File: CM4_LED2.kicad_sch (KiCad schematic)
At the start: 2 parts

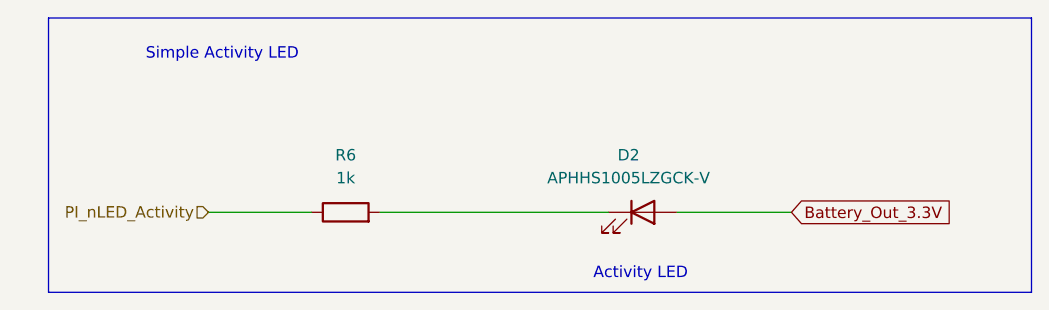
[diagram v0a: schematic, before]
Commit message: chore: Many routing changes
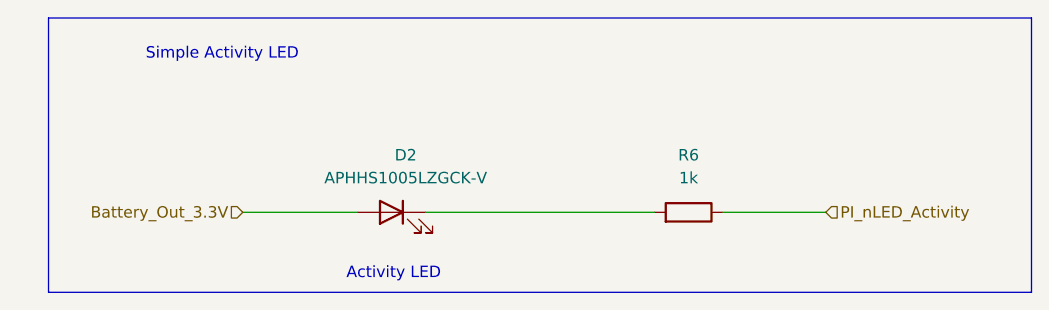
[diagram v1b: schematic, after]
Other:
- moved on the sheet: D2, R6
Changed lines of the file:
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@@
 	(text "Activity LED"
 		(exclude_from_sim no)
-		(at 119.126 69.088 0)
+		(at 91.694 69.088 0)
 		(effects
 			(font
@@
 	(wire
 		(pts
-			(xy 90.17 62.23) (xy 115.57 62.23)
+			(xy 120.65 62.23) (xy 95.25 62.23)
 		)
 		(stroke
@@
 	(wire
 		(pts
-			(xy 71.12 62.23) (xy 82.55 62.23)
+			(xy 139.7 62.23) (xy 128.27 62.23)
 		)
 		(stroke
@@
 	(wire
 		(pts
-			(xy 123.19 62.23) (xy 135.89 62.23)
+			(xy 87.63 62.23) (xy 74.93 62.23)
 		)
 		(stroke
@@
 		)
 	)
-	(global_label "Battery_Out_3.3V"
+	(hierarchical_label "PI_nLED_Activity"
 		(shape input)
-		(at 135.89 62.23 0)
-		(fields_autoplaced yes)
+		(at 139.7 62.23 0)
 		(effects
 			(font
@@
 			(justify left)
 		)
-		(property "Intersheetrefs" "${INTERSHEET_REFS}"
-			(at 154.8408 62.23 0)
-			(effects
-				(font
-					(size 1.27 1.27)
-				)
-				(justify left)
-				(hide yes)
-			)
-		)
-	)
-	(hierarchical_label "PI_nLED_Activity"
+	)
+	(hierarchical_label "Battery_Out_3.3V"
 		(shape input)
-		(at 71.12 62.23 180)
+		(at 74.93 62.23 180)
 		(effects
 			(font
@@
 	(symbol
 		(lib_id "#dzdb:g_res/R-1k-0603")
-		(at 86.36 62.23 90)
+		(at 124.46 62.23 270)
+		(mirror x)
 		(unit 1)
 		(exclude_from_sim no)
@@
 		(fields_autoplaced yes)
 		(property "Reference" "R6"
-			(at 86.36 55.88 90)
+			(at 124.46 55.88 90)
 			(effects
 				(font
@@
 		)
 		(property "Value" "1k"
-			(at 86.36 58.42 90)
+			(at 124.46 58.42 90)
 			(effects
 				(font
@@
 		)
 		(property "Footprint" "Resistor_SMD:R_0603_1608Metric"
-			(at 86.36 64.008 90)
+			(at 124.46 64.008 90)
 			(effects
 				(font
@@
 		)
 		(property "Datasheet" "https://www.we-online.com/components/products/datasheet/560112116014.pdf"
-			(at 86.36 62.23 0)
+			(at 124.46 62.23 0)
 			(effects
 				(font
@@
 		)
 		(property "Description" "Thick Film Resistors - SMD WRIS-RSKS 1 kOhms 1 % 0.1 W 0603"
-			(at 86.36 62.23 0)
+			(at 124.46 62.23 0)
 			(effects
 				(font
@@
 		)
 		(property "IPN" "R-1k-0603"
-			(at 86.36 62.23 0)
+			(at 124.46 62.23 0)
 			(effects
 				(font
@@
 		)
 		(property "MPN" "560112116014"
-			(at 86.36 62.23 0)
+			(at 124.46 62.23 0)
 			(effects
 				(font
@@
 		)
 		(property "Manufacturer" "Wurth Elektronik"
-			(at 86.36 62.23 0)
+			(at 124.46 62.23 0)
 			(effects
 				(font
@@
 		)
 		(property "Resistance" "1k"
-			(at 86.36 62.23 0)
+			(at 124.46 62.23 0)
 			(effects
 				(font
@@
 		)
 		(property "Power" "0.1 W"
-			(at 86.36 62.23 0)
+			(at 124.46 62.23 0)
 			(effects
 				(font
@@
 		)
 		(property "Material" "Thick film"
-			(at 86.36 62.23 0)
+			(at 124.46 62.23 0)
 			(effects
 				(font
@@
 		)
 		(property "Tolerance" "1 %"
-			(at 86.36 62.23 0)
+			(at 124.46 62.23 0)
 			(effects
 				(font
@@
 		)
 		(property "Supplier" "Mouser"
-			(at 86.36 62.23 0)
+			(at 124.46 62.23 0)
 			(effects
 				(font
@@
 		)
 		(property "SPN" "710-560112116014"
-			(at 86.36 62.23 0)
+			(at 124.46 62.23 0)
 			(effects
 				(font
@@
 		)
 		(property "LCSC" "CXXXXX"
-			(at 86.36 62.23 0)
+			(at 124.46 62.23 0)
 			(effects
 				(font
@@
 		)
 		(property "Comment" "lifecycle=Active; note=Auto-generated"
-			(at 86.36 62.23 0)
+			(at 124.46 62.23 0)
 			(effects
 				(font
@@
 	(symbol
 		(lib_id "#dzdb:s_dio/D-KIN-APHHS1005LZGCK-V")
-		(at 119.38 62.23 0)
+		(at 91.44 62.23 0)
+		(mirror y)
 		(unit 1)
 		(exclude_from_sim no)
@@
 		(fields_autoplaced yes)
 		(property "Reference" "D2"
-			(at 117.7925 55.88 0)
+			(at 93.0275 55.88 0)
 			(effects
 				(font
@@
 		)
 		(property "Value" "APHHS1005LZGCK-V"
-			(at 117.7925 58.42 0)
+			(at 93.0275 58.42 0)
 			(effects
 				(font
@@
 		)
 		(property "Footprint" "LED_SMD:LED_0402_1005Metric"
-			(at 119.38 62.23 0)
+			(at 91.44 62.23 0)
 			(effects
 				(font
@@
 		)
 		(property "Datasheet" "https://www.kingbrightusa.com/images/catalog/SPEC/APHHS1005LZGCK-V.pdf"
-			(at 119.38 62.23 0)
+			(at 91.44 62.23 0)
 			(effects
 				(font
@@
 		)
 		(property "Description" "LED EMERALD GREEN 525nm 180mcd@2mA 40mcd@0.44mA 2.54V"
-			(at 119.38 62.23 0)
+			(at 91.44 62.23 0)
 			(effects
 				(font
@@
 		)
 		(property "Sim.Pins" "1=K 2=A"
-			(at 119.38 62.23 0)
+			(at 91.44 62.23 0)
 			(effects
 				(font
@@
 		)
 		(property "IPN" "D-KIN-APHHS1005LZGCK-V"
-			(at 119.38 62.23 0)
+			(at 91.44 62.23 0)
 			(effects
 				(font
@@
 		)
 		(property "MPN" "APHHS1005LZGCK-V"
-			(at 119.38 62.23 0)
+			(at 91.44 62.23 0)
 			(effects
 				(font
@@
 		)
 		(property "Manufacturer" "Kingbright"
-			(at 119.38 62.23 0)
+			(at 91.44 62.23 0)
 			(effects
 				(font
@@
 		)
 		(property "Type" "LED GREEN"
-			(at 119.38 62.23 0)
+			(at 91.44 62.23 0)
 			(effects
 				(font
@@
 		)
 		(property "Vf" "2.65V"
-			(at 119.38 62.23 0)
+			(at 91.44 62.23 0)
 			(effects
 				(font
@@
 		)
 		(property "If" "2mA"
-			(at 119.38 62.23 0)
+			(at 91.44 62.23 0)
 			(effects
 				(font
@@
 		)
 		(property "Supplier" "Mouser"
-			(at 119.38 62.23 0)
+			(at 91.44 62.23 0)
 			(effects
 				(font
@@
 		)
 		(property "SPN" "604-APHHS1005LZGCK-V"
-			(at 119.38 62.23 0)
+			(at 91.44 62.23 0)
 			(effects
 				(font
@@
 		)
 		(property "LCSC" "C5875752"
-			(at 119.38 62.23 0)
+			(at 91.44 62.23 0)
 			(effects
 				(font
@@
 		)
 		(property "Comment" "lifecycle=Active"
-			(at 119.38 62.23 0)
-			(effects
-				(font
+			(at 91.44 62.23 0)
+			(effects
+				(font

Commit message: chore: more cleanup
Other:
- company: (none) -> Davide
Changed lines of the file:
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@@
 	(generator_version "9.0")
 	(paper "A4")
+	(title_block
+		(date "2025-11-18")
+		(company "Davide")
+	)
 	(rectangle
 		(start 53.34 40.64)
